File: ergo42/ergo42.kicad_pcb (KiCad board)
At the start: 2 copper layers, 91.4 x 54.6 mm, 10 parts, among them SW1 SW_PUSH, SW13 SW_PUSH, SW29 SW_Push, SW5 SW_PUSH, SW9 SW_PUSH, U3 ProMicro

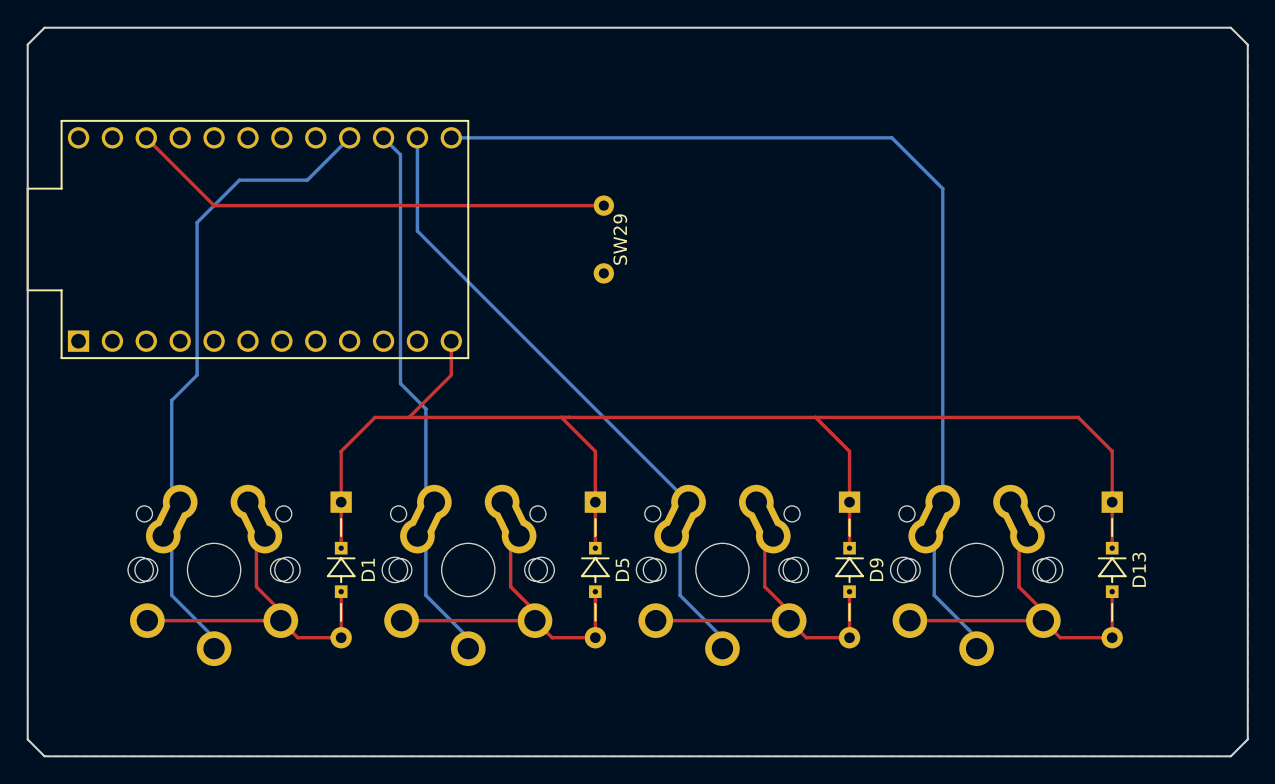
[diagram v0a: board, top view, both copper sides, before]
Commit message: Implement
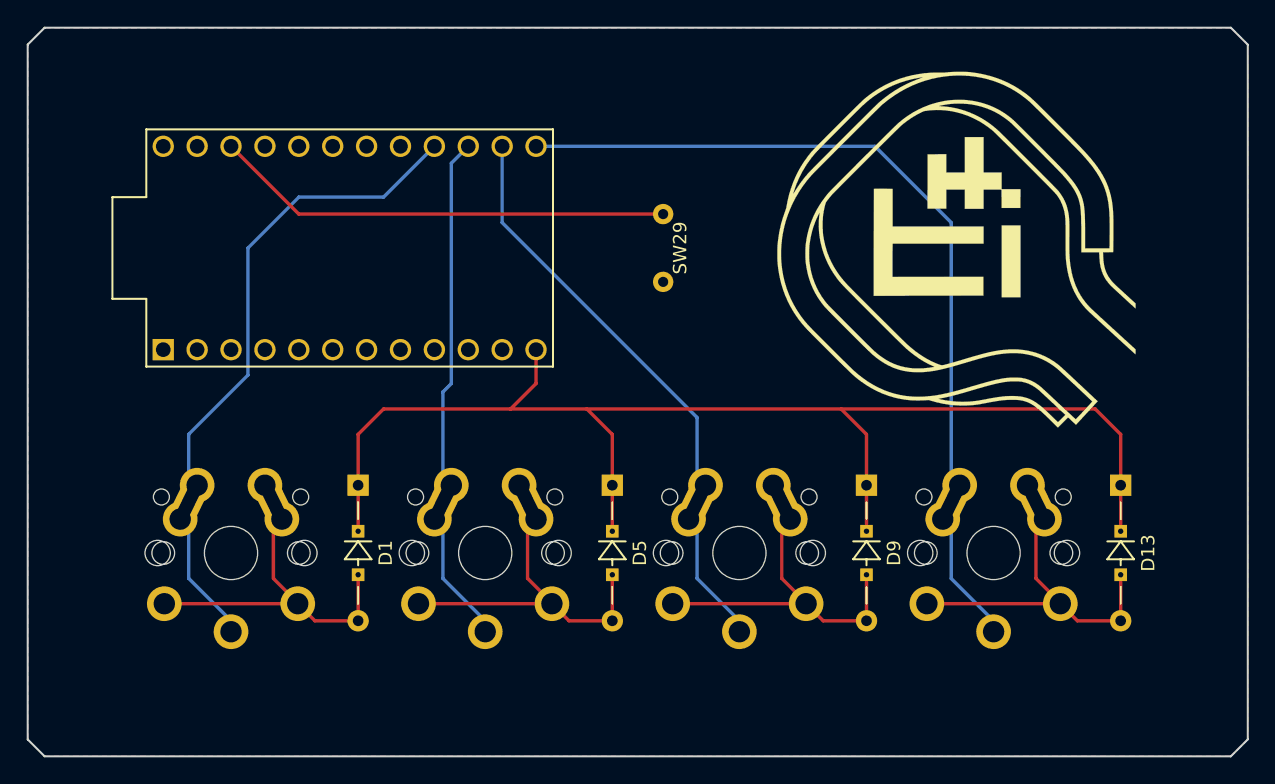
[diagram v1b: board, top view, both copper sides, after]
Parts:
- added G***: LOGO, library:biacco42, F.Cu at (142.2, 103.5)
- added G***: LOGO, library:tanoshii_life, B.Cu at (142.9, 106.7)
- moved U3 6.38 mm to (97.8, 104.1)
- moved SW29 4.49 mm to (121.3, 104.1)
- moved SW1 1.80 mm to (88.9, 127.0)
- moved SW13 1.80 mm to (146.1, 127.0)
- moved D9 1.80 mm to (136.5, 121.9)
- moved SW5 1.80 mm to (108.0, 127.0)
- moved SW9 1.80 mm to (127.0, 127.0)
- moved D1 1.80 mm to (98.4, 121.9)
- moved D5 1.80 mm to (117.5, 121.9)
- moved D13 1.42 mm to (155.6, 121.9)
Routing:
- net /col3: track 74.3 -> 65.5 mm
- net /row0: track 103.8 -> 98.4 mm
- net /col2: track 48.2 -> 43.7 mm
- net /col1: track 40.9 -> 38.5 mm
- net /rst: track 36.4 -> 34.5 mm
- net /col0: track 48.1 -> 49.0 mm
- net Net-(D9-Pad2): track 26.9 -> 27.6 mm
- net Net-(D5-Pad2): track 26.9 -> 27.6 mm
- net Net-(D1-Pad2): track 26.9 -> 27.6 mm
